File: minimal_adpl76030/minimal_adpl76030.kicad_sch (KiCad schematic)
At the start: 1 part, among them U1 ADPL76030EUFD-PBF

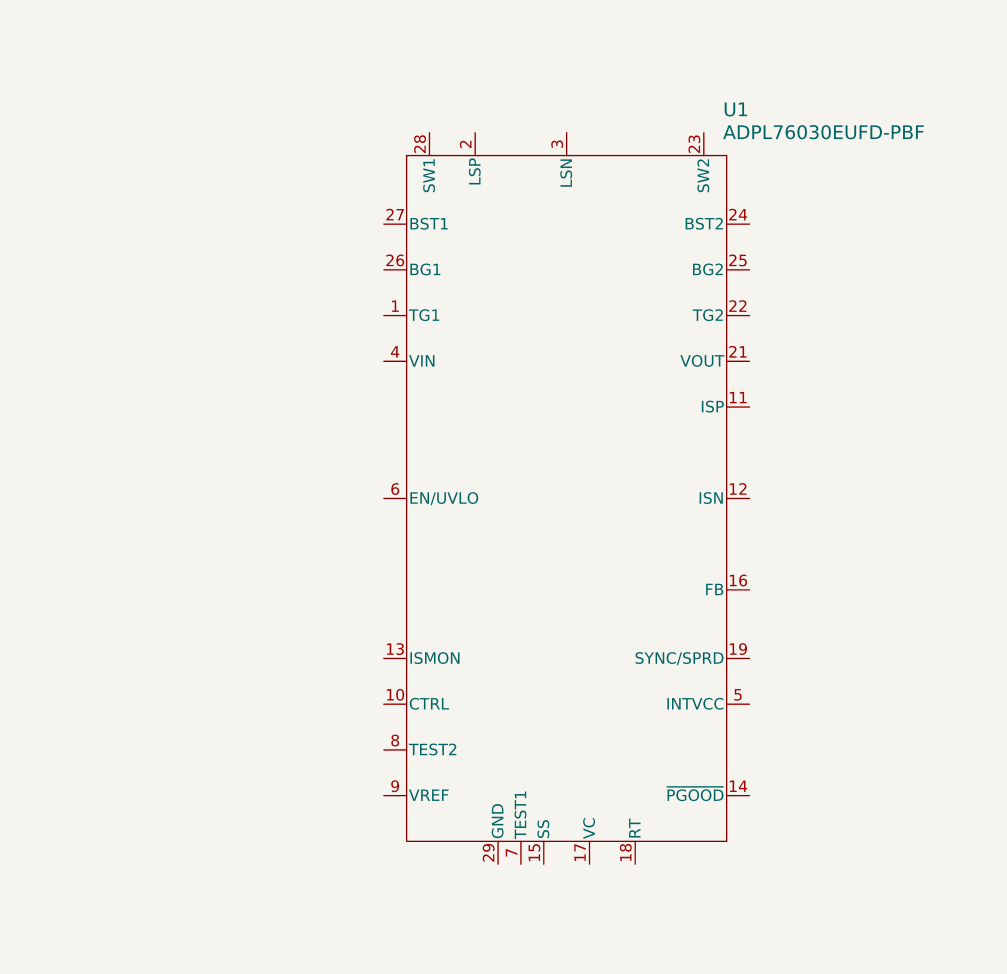
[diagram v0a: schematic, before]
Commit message: backup
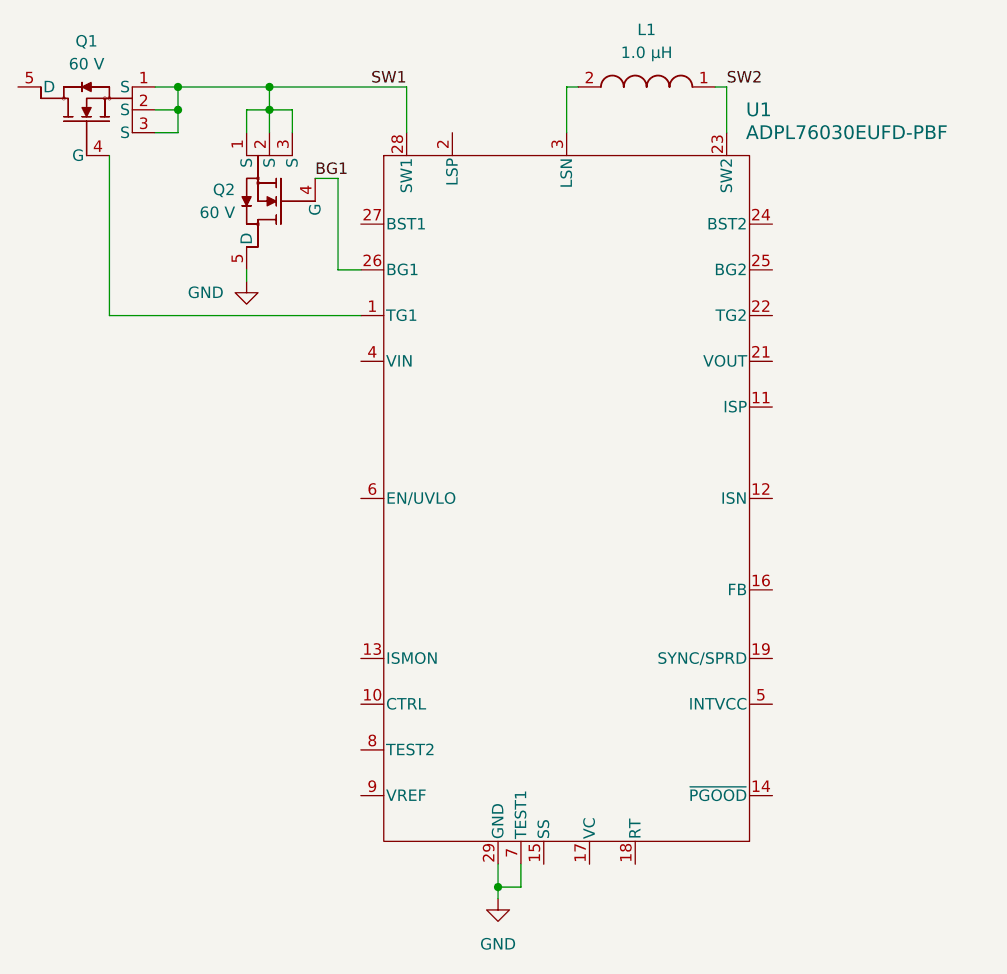
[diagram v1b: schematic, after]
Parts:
- added L1: 1.0 µH, inductor_footprints:74437336, symbol INDUCTORS_74437336_DATA_BASE:L_74437336010
- added Q1, Q2: 60 V, transistor_footprints:TSDSON-8FL, symbol TRANSISTORS_BSZ065N06LS5ATMA1_DATA_BASE:Q_BSZ065N06LS5ATMA1
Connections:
- net at U1.1 (TG1): now also Q1.4 (G)
- net SW2: now reaches U1.23 (SW2)
- net SW2: now also L1.1
- net BG1: now reaches U1.26 (BG1)
- net BG1: now also Q2.4 (G)
- net SW1: now reaches U1.28 (SW1)
- net SW1: now also Q1.1 (S), Q1.2 (S), Q1.3 (S), Q2.1 (S), Q2.2 (S), Q2.3 (S)
- net GND: now reaches U1.29 (GND)
- net GND: now also U1.7 (TEST1), Q2.5 (D)
- net at U1.3 (LSN): now also L1.2
